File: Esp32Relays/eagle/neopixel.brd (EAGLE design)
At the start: 54.4 x 16.6 mm, 20 parts, among them J1 Audio2, J3 AUDIO_JACK_3.5MM_PTH, J4 AUDIO_JACK_3.5MM_PTH, U1 CD4066BE

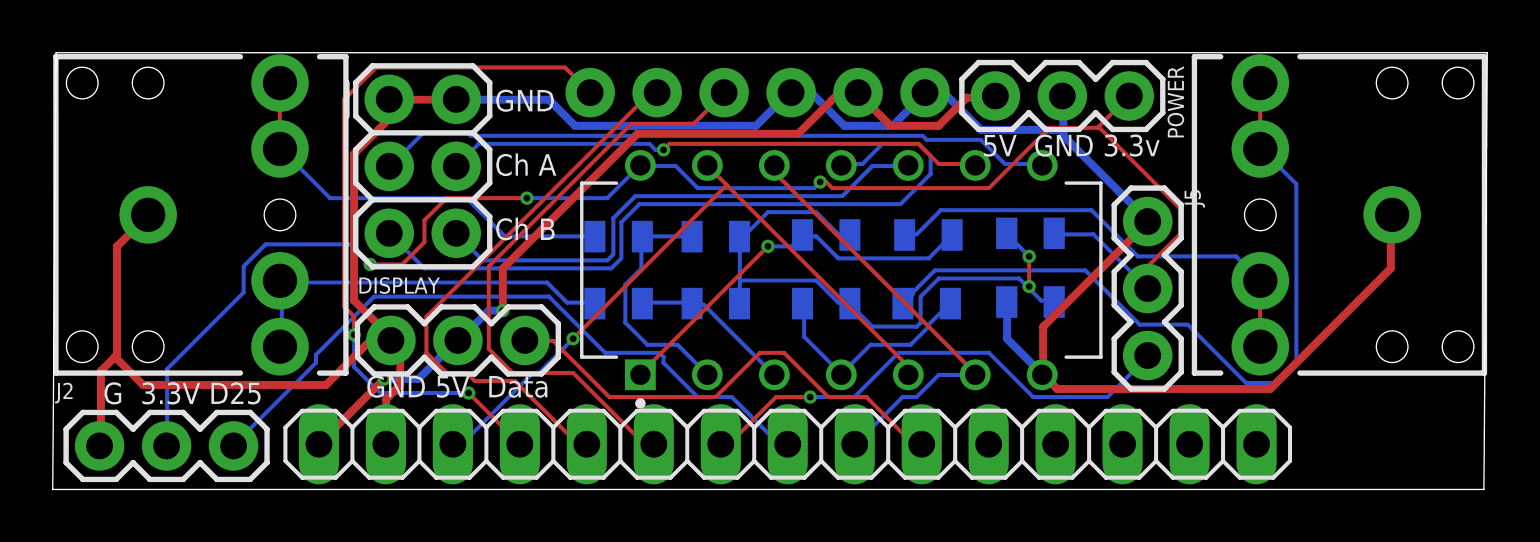
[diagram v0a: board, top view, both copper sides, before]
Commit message: Schematic update
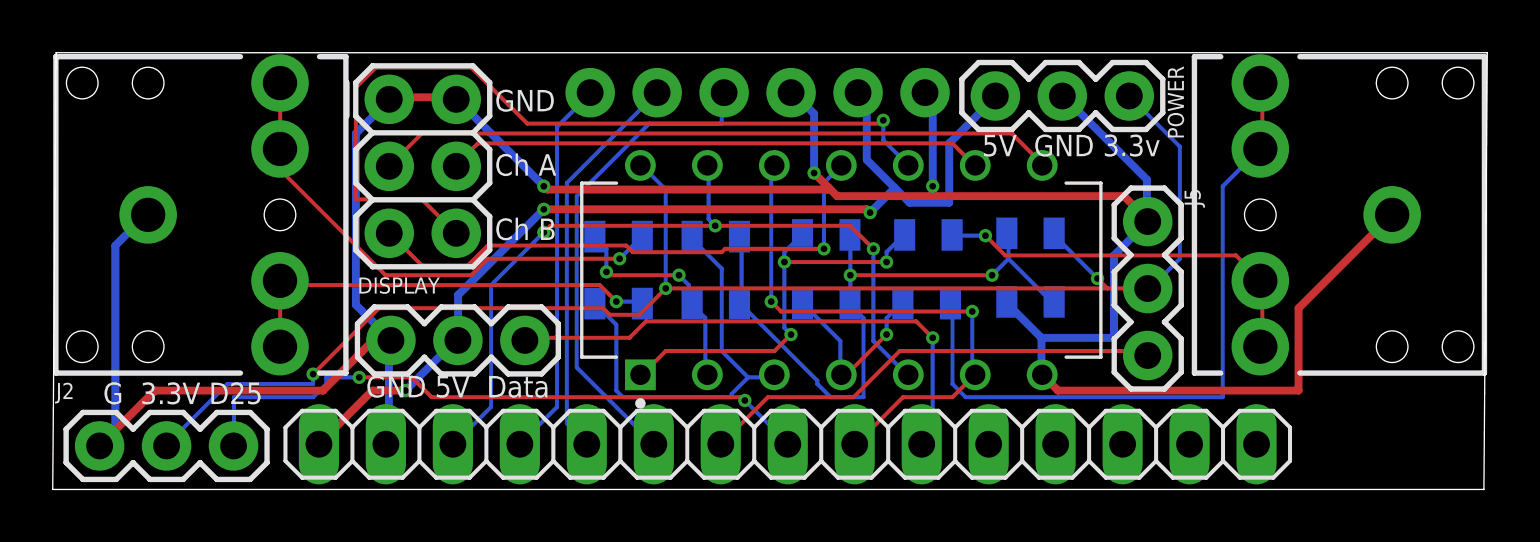
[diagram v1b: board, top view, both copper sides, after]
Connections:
- net A1-SIG-IN: now also C1.2; no longer C1.1
- net A1-SIG-OUT: now also C4.2, R6.2; no longer C4.1, R5.2
- net A1IN: now also C1.1; no longer C1.2
- net A1OUT: now also C4.1; no longer C4.2
- net B1-SIG-IN: now also C3.2; no longer C3.1
- net B1-SIG-OUT: now also C5.2, R5.2; no longer C5.1, R6.2
- net B1IN: now also C3.1; no longer C3.2
- net B1OUT: now also C5.1; no longer C5.2
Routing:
- net D12: track 28.0 -> 14.4 mm, vias 2 -> 0
- net GND: track 98.4 -> 110.9 mm, vias 0 -> 3
- net B2OUT: track 19.9 -> 31.9 mm, vias 0 -> 1
- net B1-SIG-OUT: track 6.16 -> 16.4 mm
- net B2IN: track 28.0 -> 20.9 mm, vias 0 -> 1
- net D14: track 21.2 -> 15.1 mm
- net VIN: track 33.1 -> 38.2 mm, vias 2 -> 3
- net D13: track 25.5 -> 30.2 mm, vias 1 -> 3
- net D33: track 16.8 -> 21.2 mm, vias 0 -> 2
- net D27: track 22.6 -> 18.5 mm
- net A1OUT: track 15.8 -> 19.3 mm, vias 0 -> 1
- net B1IN: track 28.7 -> 26.1 mm
- net A1IN: track 17.5 -> 15.0 mm, vias 0 -> 1
- net D32: track 18.1 -> 20.2 mm, vias 0 -> 1
- net 3V3: track 58.6 -> 56.8 mm
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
